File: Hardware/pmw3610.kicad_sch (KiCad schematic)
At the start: 11 parts, among them U2 PMW3610DM-SUDU, U3 TLV74318P

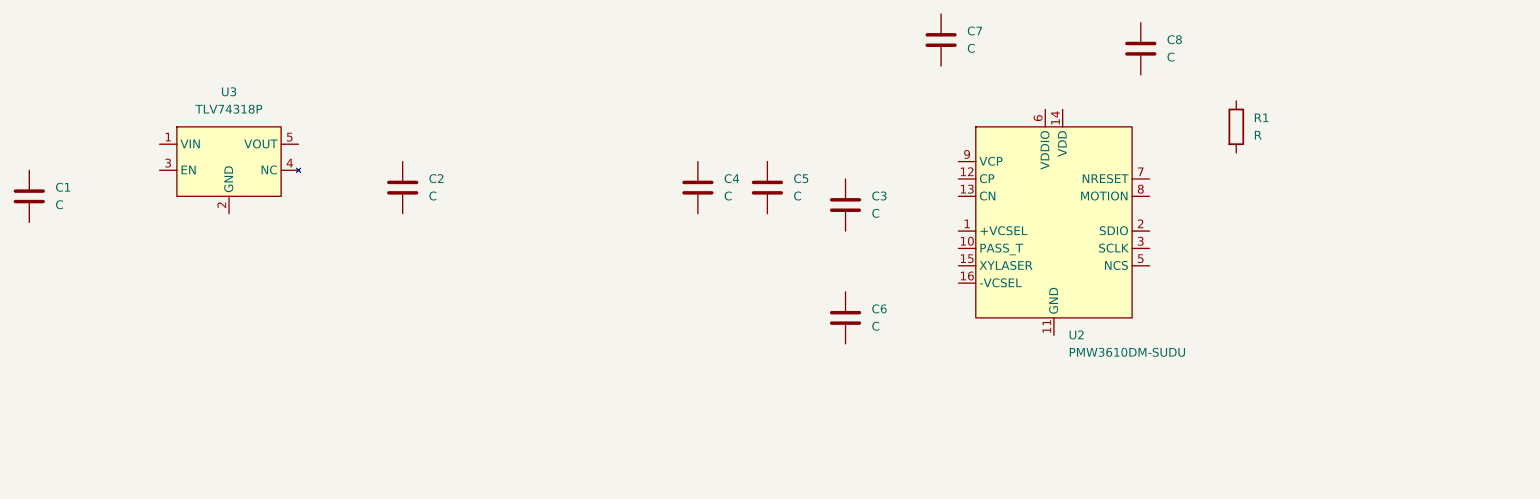
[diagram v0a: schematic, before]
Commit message: update the schematics
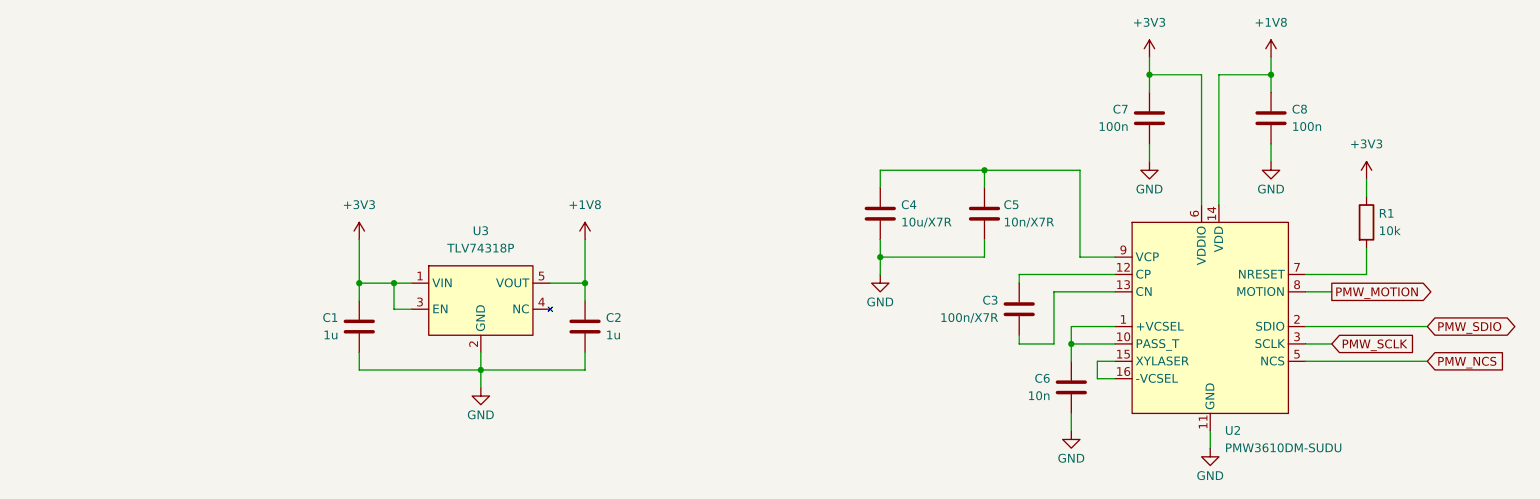
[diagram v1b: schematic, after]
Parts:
- C1, C2: value C -> 1u; footprint (none) -> Adept_BLE_footprints:C_0805
- C3: value C -> 100n/X7R; footprint (none) -> Adept_BLE_footprints:C_0805
- C4: value C -> 10u/X7R; footprint (none) -> Adept_BLE_footprints:C_0805
- C5: value C -> 10n/X7R; footprint (none) -> Adept_BLE_footprints:C_0805
- C6: value C -> 10n; footprint (none) -> Adept_BLE_footprints:C_0805
- C7, C8: value C -> 100n; footprint (none) -> Adept_BLE_footprints:C_0805
- R1: value R -> 10k; footprint (none) -> Adept_BLE_footprints:R_0805
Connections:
- net +3V3: now reaches C7.1
- net +3V3: now also C1.1, R1.1, U2.6 (VDDIO), U3.1 (VIN), U3.3 (EN)
- net GND: now reaches C7.2
- net GND: now also C1.2, C2.2, C4.2, C5.2, C6.2, C8.2, U2.11 (GND), U3.2 (GND)
- net at C6.1: now also U2.1 (+VCSEL), U2.10 (PASS_T)
- net +1V8: now reaches U3.5 (VOUT)
- net +1V8: now also C2.1, C8.1, U2.14 (VDD)
- net at C4.1: now also C5.1, U2.9 (VCP)
- net at C3.1: now also U2.12 (CP)
- net at C3.2: now also U2.13 (CN)
- net at U2.15 (XYLASER): now also U2.16 (-VCSEL)
- net PMW_SDIO: now reaches U2.2 (SDIO)
- net PMW_SCLK: now reaches U2.3 (SCLK)
- net PMW_NCS: now reaches U2.5 (NCS)
- net at U2.7 (NRESET): now also R1.2
- net PMW_MOTION: now reaches U2.8 (MOTION)
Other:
- moved on the sheet: C1, C2, C3, C4, C5, C6, C7, C8, R1, U2, U3
